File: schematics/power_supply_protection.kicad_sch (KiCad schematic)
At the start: 29 parts, among them J1 Conn_01x01_Pin, J2 ATX-20, J3 Conn_01x05_MountingPin, J4 Conn_01x05_MountingPin, K1 FINDER-40.31, Q1 BC557, Q2 BD139, Q3 BC547, Q4 BC547, Q5 BC547, Q6 BC547, Q7 BC547, Q8 BC547, SW1 SW_DPST_x2, SW2 SW_Push

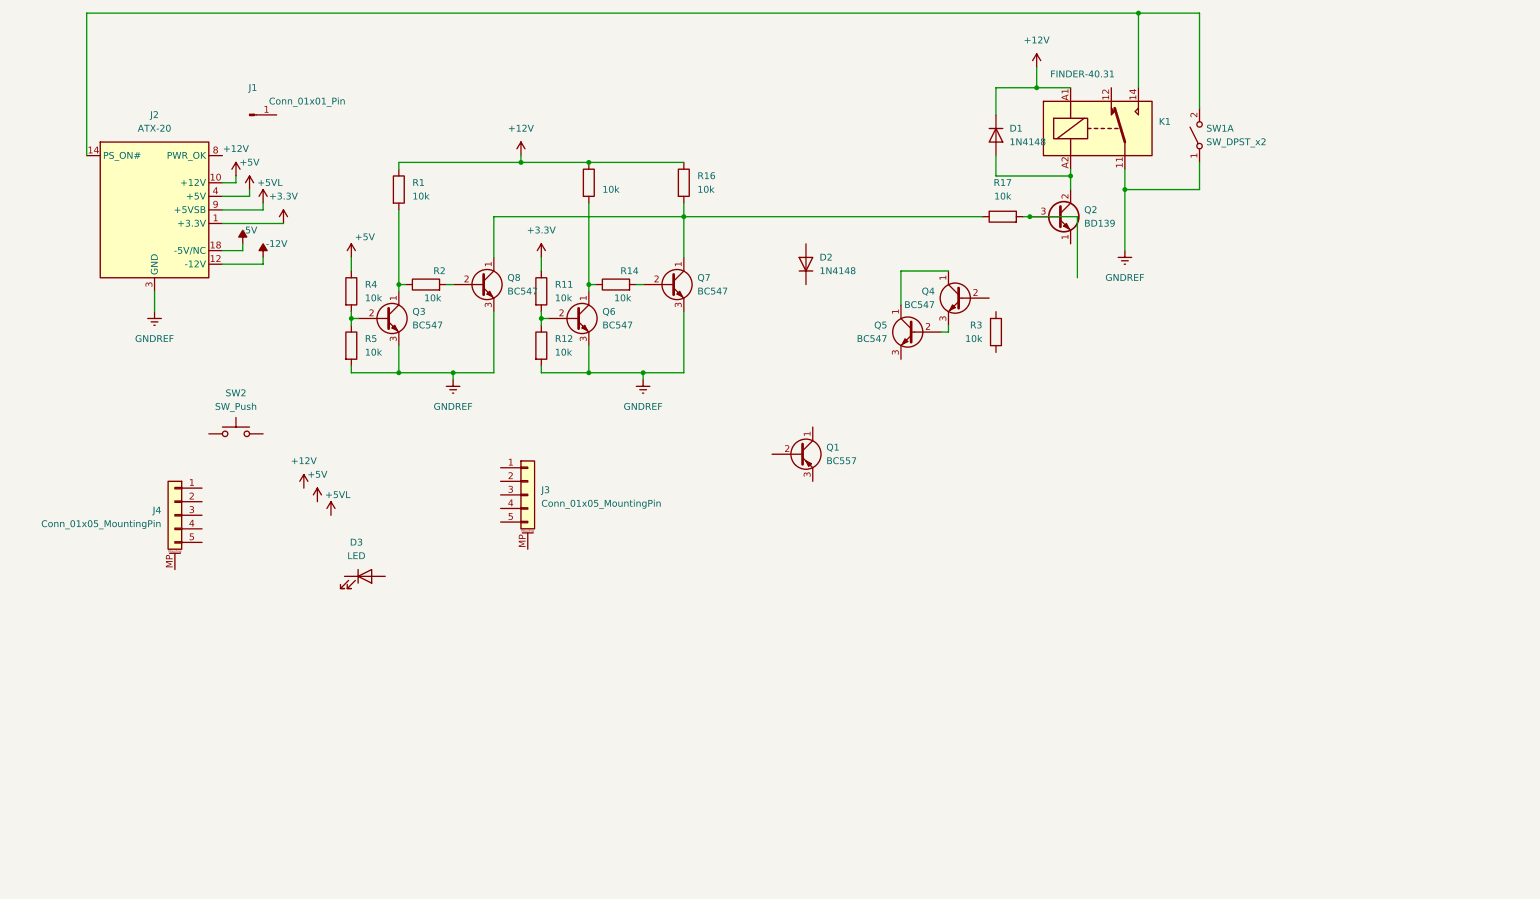
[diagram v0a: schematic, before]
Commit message: finished 1.0
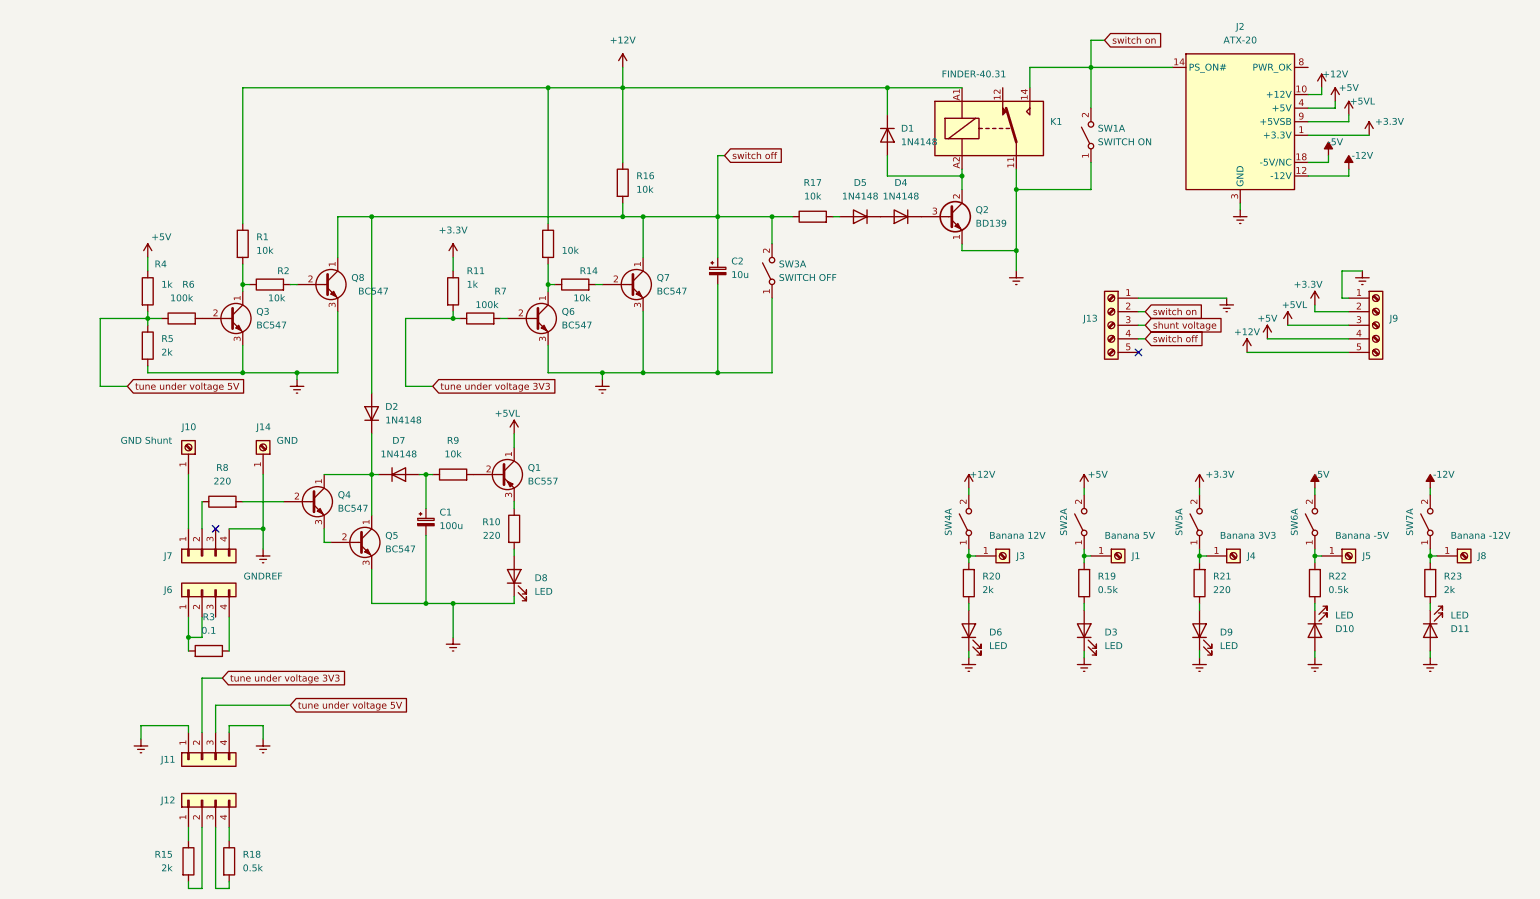
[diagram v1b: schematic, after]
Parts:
- removed J1: Conn_01x01_Pin, symbol Connector:Conn_01x01_Pin
- removed J3, J4: Conn_01x05_MountingPin, symbol Connector_Generic_MountingPin:Conn_01x05_MountingPin
- removed R12: 10k, symbol Device:R
- removed SW2: SW_Push, symbol Switch:SW_Push
- added C1: 100u, symbol Device:C_Polarized_Small
- added C2: 10u, symbol Device:C_Polarized_Small
- added D10, D11, D6, D8, D9: LED, symbol Device:LED
- added D4, D5, D7: 1N4148, Diode_THT:D_DO-35_SOD27_P7.62mm_Horizontal, symbol Diode:1N4148
- added J1: Banana 5V, symbol Connector:Screw_Terminal_01x01
- added J10: GND Shunt, symbol Connector:Screw_Terminal_01x01
- added J11, J12, J6, J7: Conn_01x04, symbol Connector_Generic:Conn_01x04
- added J13, J9: Screw_Terminal_01x05, symbol Connector:Screw_Terminal_01x05
- added J14: GND, symbol Connector:Screw_Terminal_01x01
- added J3: Banana 12V, symbol Connector:Screw_Terminal_01x01
- added J4: Banana 3V3, symbol Connector:Screw_Terminal_01x01
- added J5: Banana -5V, symbol Connector:Screw_Terminal_01x01
- added J8: Banana -12V, symbol Connector:Screw_Terminal_01x01
- added R10, R21, R8: 220, symbol Device:R
- added R15, R20, R23: 2k, symbol Device:R
- added R18, R19, R22: 0.5k, symbol Device:R
- added R6, R7: 100k, symbol Device:R
- added R9: 10k, symbol Device:R
- added SW2, SW4, SW5, SW6, SW7: SW_DPST_x2, symbol Switch:SW_DPST_x2
- added SW3: SWITCH OFF, symbol Switch:SW_DPST_x2
- R11, R4: value 10k -> 1k
- R3: value 10k -> 0.1
- R5: value 10k -> 2k
- SW1: value SW_DPST_x2 -> SWITCH ON
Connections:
- net +12V: now also J9.5 (Pin_5), SW4.2 (B)
- net +3.3V: now also J9.2 (Pin_2), SW5.2 (B)
- net +5V: now also J9.4 (Pin_4), SW2.2 (B)
- net +5VL: now also Q1.1 (C), J9.3 (Pin_3)
- net -12V: now also SW7.2 (B)
- net -5V: now also SW6.2 (B)
- net GNDREF: now also D3.1 (K), Q2.1 (E), Q5.3 (E), C1.2, C2.2, D10.2 (A), D11.2 (A), D6.1 (K), D8.1 (K), D9.1 (K), J11.1 (Pin_1), J11.4 (Pin_4), J13.1 (Pin_1), J14.1 (Pin_1), J7.4 (Pin_4), J9.1 (Pin_1), SW3.1 (A)
- net at Q1.2 (B): now also R9.2
- net at Q1.3 (E): now also R10.1
- net at D2.1 (K): now also Q4.1 (C), Q5.1 (C), D7.1 (K)
- net switch off: now reaches D2.2 (A)
- net switch off: now also Q7.1 (C), Q8.1 (C), R16.2, R17.1, C2.1, J13.4 (Pin_4), SW3.2 (B)
- net at D3.2 (A): now also R19.1
- net tune under voltage 5V: now reaches R4.2, R5.1
- net tune under voltage 5V: now also J11.3 (Pin_3), R6.1; no longer Q3.2 (B)
- net at Q6.2 (B): now also R7.2; no longer R11.2
- net switch on: now reaches J2.14 (PS_ON#), K1.14, SW1.2 (B)
- net switch on: now also J13.2 (Pin_2)
- net at Q2.3 (B): now also D4.1 (K); no longer R17.2
- net at Q4.2 (B): now also R8.2
- net at R3.1: now also J6.4 (Pin_4)
- net at R3.2: now also J6.1 (Pin_1), J6.2 (Pin_2)
- new net: D6.2 (A), R20.1
- new net: J8.1 (Pin_1), R23.2, SW7.1 (A)
- new net: C1.1, D7.2 (A), R9.1
- new net: J4.1 (Pin_1), R21.2, SW5.1 (A)
- new net: J3.1 (Pin_1), R20.2, SW4.1 (A)
- new net: D9.2 (A), R21.1
- new net: D11.1 (K), R23.1
- new net: J12.1 (Pin_1), R15.1
- new net: J12.2 (Pin_2), R15.2
- new net: J12.3 (Pin_3), R18.2
- new net: J12.4 (Pin_4), R18.1
- new net: D8.2 (A), R10.2
- new net: J5.1 (Pin_1), R22.2, SW6.1 (A)
- new net: D4.2 (A), D5.1 (K)
- new net: D5.2 (A), R17.2
- new net: Q3.2 (B), R6.2
- new net: J1.1 (Pin_1), R19.2, SW2.1 (A)
- new net: J7.2 (Pin_2), R8.1
- new net: D10.1 (K), R22.1
- new net: J10.1 (Pin_1), J7.1 (Pin_1)
- new net shunt voltage: J13.3 (Pin_3)
- new net tune under voltage 3V3: J11.2 (Pin_2), R11.2, R7.1
- no-connect marks 0 -> 2
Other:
- company: (none) -> Jonatan Asensio Palao
- title: (none) -> Voltage and current protection for ATX power supply
- moved on the sheet: D1, J2, K1, Q1, Q2, Q3, Q4, Q5, Q6, Q7, Q8, R1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
